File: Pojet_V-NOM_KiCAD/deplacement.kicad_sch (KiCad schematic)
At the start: 8 parts, among them J301 Conn_01x06, J302 Conn_01x06, U301 ZXBM5210-SP, U302 ZXBM5210-SP

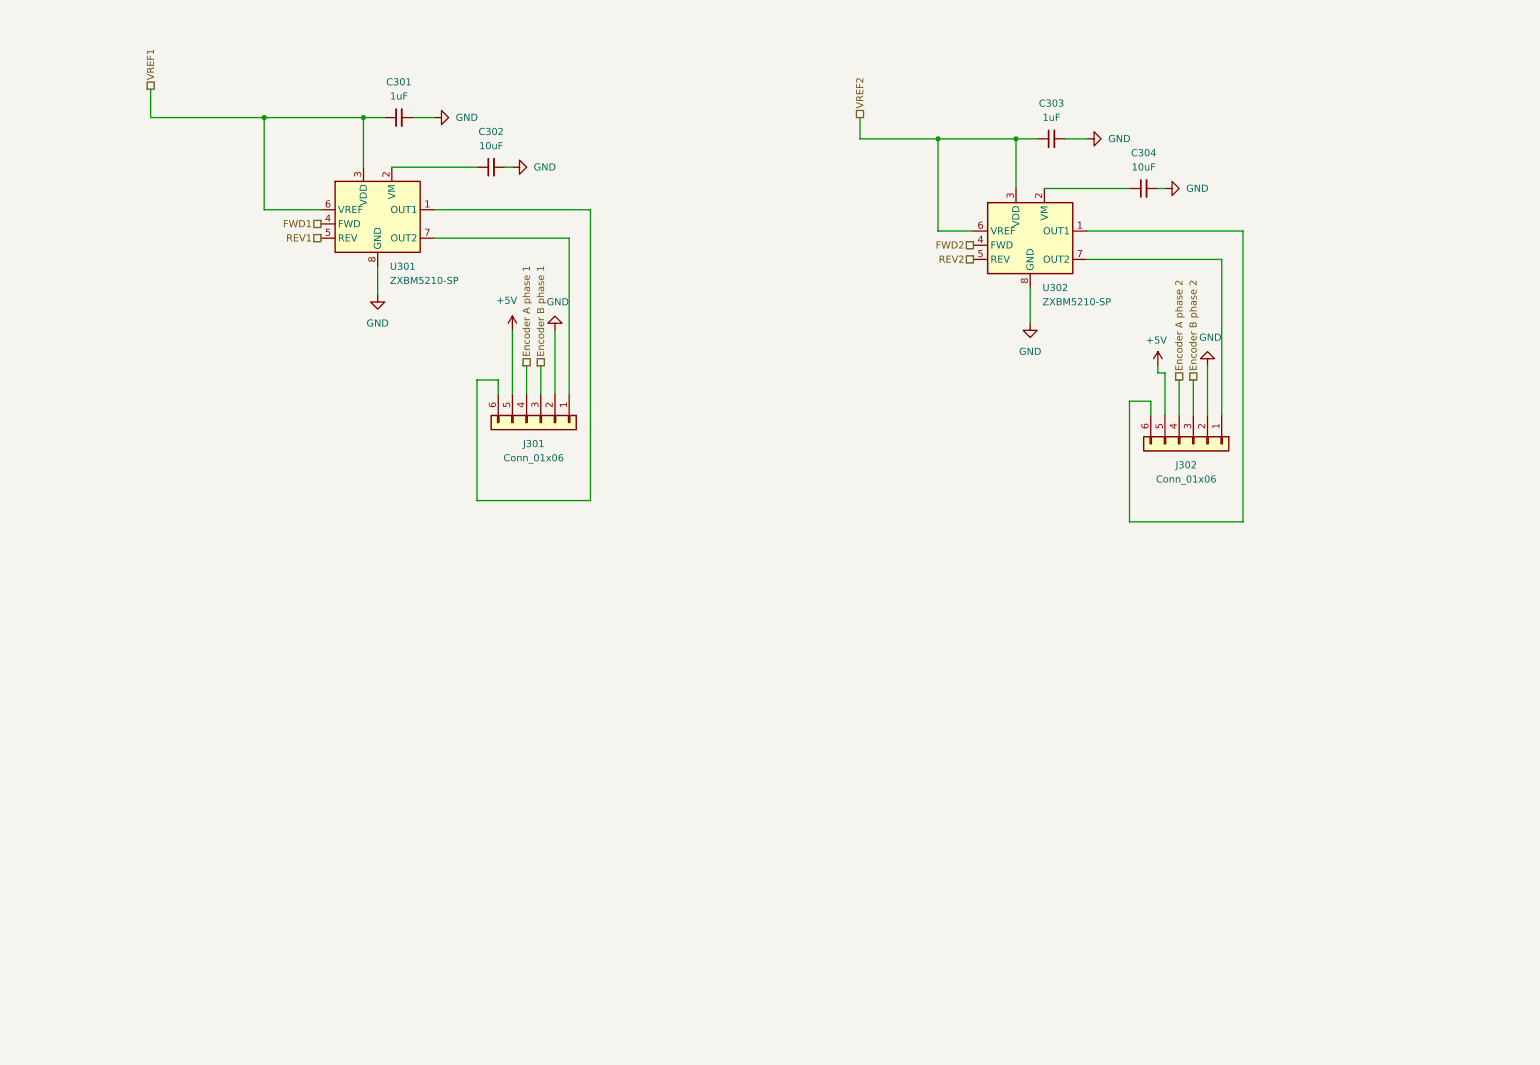
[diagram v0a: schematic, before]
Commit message: Maj Deplacement
Maj Deplacement
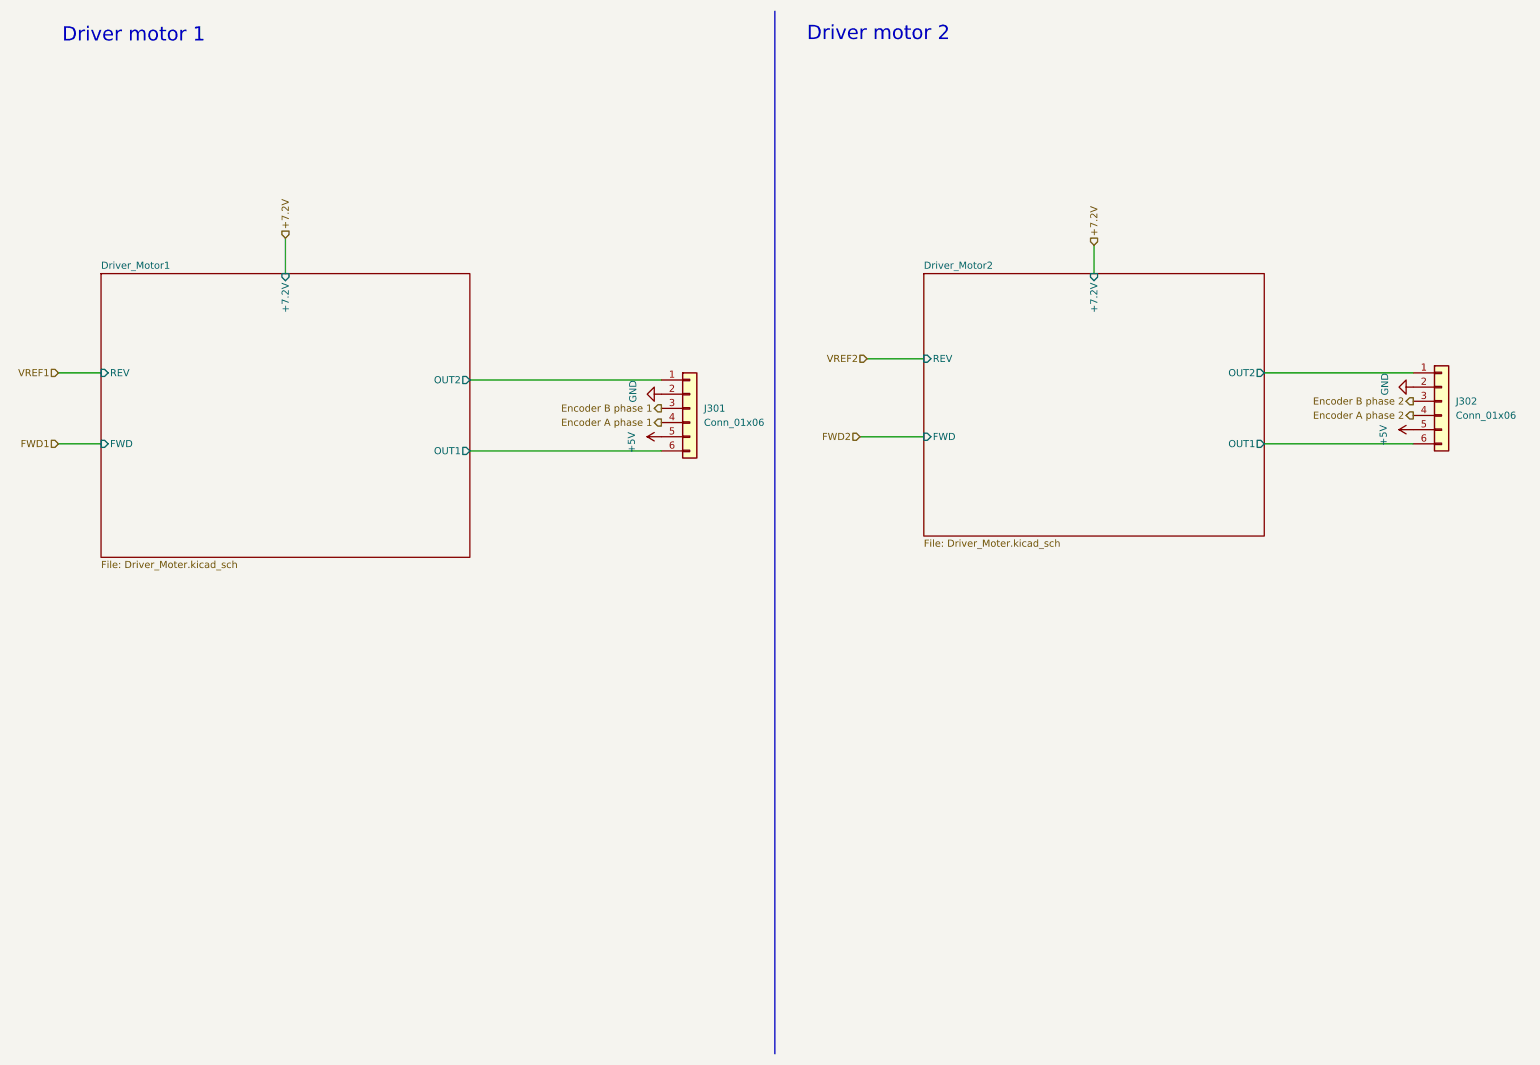
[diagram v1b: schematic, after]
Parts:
- removed C301, C303: 1uF, Capacitor_SMD:C_0402_1005Metric, symbol Device:C_Small
- removed C302, C304: 10uF, Capacitor_SMD:C_0402_1005Metric, symbol Device:C_Small
- removed U301, U302: ZXBM5210-SP, Package_SO:Diodes_SO-8EP, symbol Driver_Motor:ZXBM5210-SP
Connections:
- net Driver_Motor1/OUT1: now reaches J301.6 (Pin_6)
- net Driver_Motor1/OUT2: now reaches J301.1 (Pin_1)
- net Driver_Motor2/OUT2: now reaches J302.1 (Pin_1)
- net Driver_Motor2/OUT1: now reaches J302.6 (Pin_6)
- net Encoder A phase 1  renamed Encoder A phase 1
- net Encoder B phase 1  renamed Encoder B phase 1
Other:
- added sheet Driver_Motor1 (Driver_Moter.kicad_sch)
- added sheet Driver_Motor2 (Driver_Moter.kicad_sch)
- note added: "Driver motor 1"
- note added: "Driver motor 2"
